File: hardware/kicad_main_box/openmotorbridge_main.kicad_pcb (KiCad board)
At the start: 4 copper layers, 85 x 55 mm, 41 parts, among them J1 DEUTSCH_DTM12_IDC_HEADER, J2 MicroSD_Card, J3 USB2_IDC_HEADER_9PIN, J4 RGB_LED_3PIN, J5 PWR_BAT_NTC_4PIN, SW1 SW_PAIR_RESET, U1 LM5164-Q1, U10 SX1262IMLTRT, U11 TPS7A0533_LDO, U2 ESP32-S3-WROOM-1U-N16R8, U3 ES8388_Codec, U5 BMI270_IMU, U6 TCAN334G, U8 DW3110, U9 QCC3084_BT54_AUDIO, Y1_UWB 38.4MHz

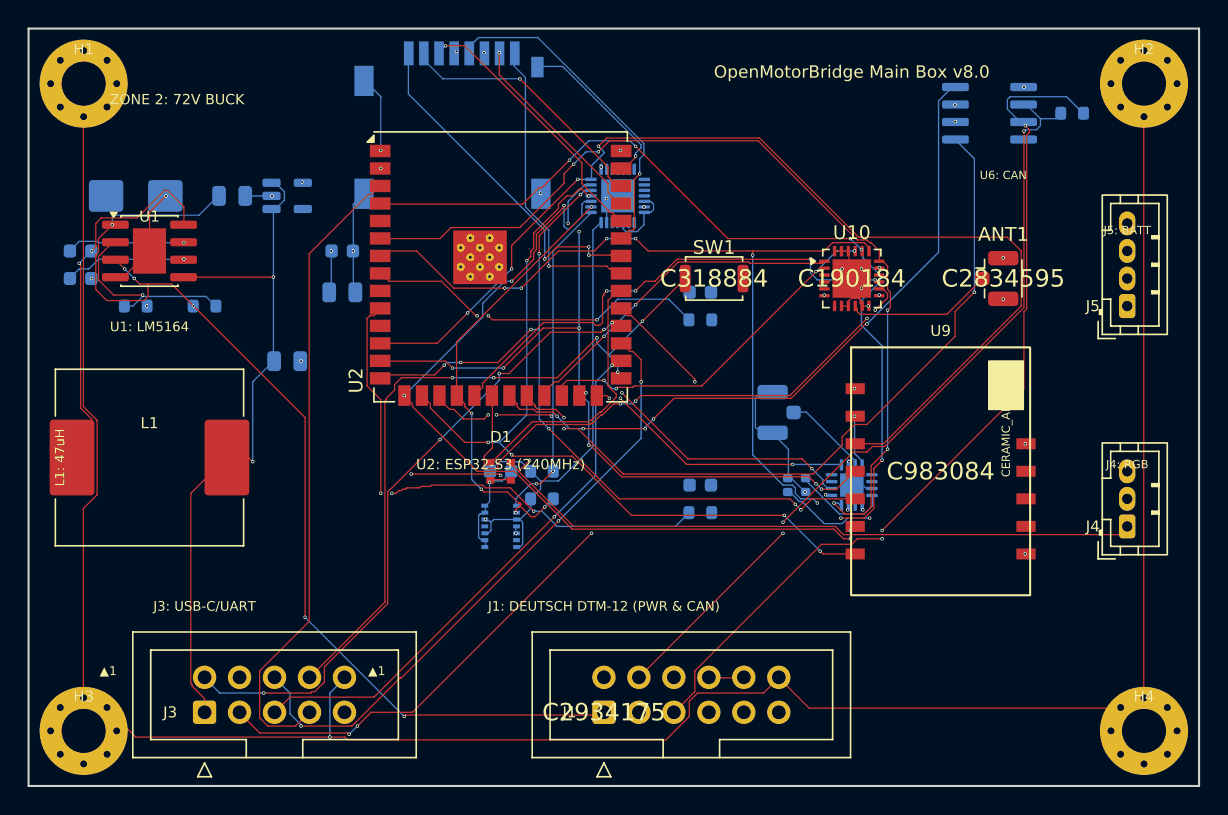
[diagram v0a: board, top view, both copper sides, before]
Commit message: feat: sync re-routed PCBAs (01, 03, 07, 08, 10), manufacturing packages, 3D renders & docs
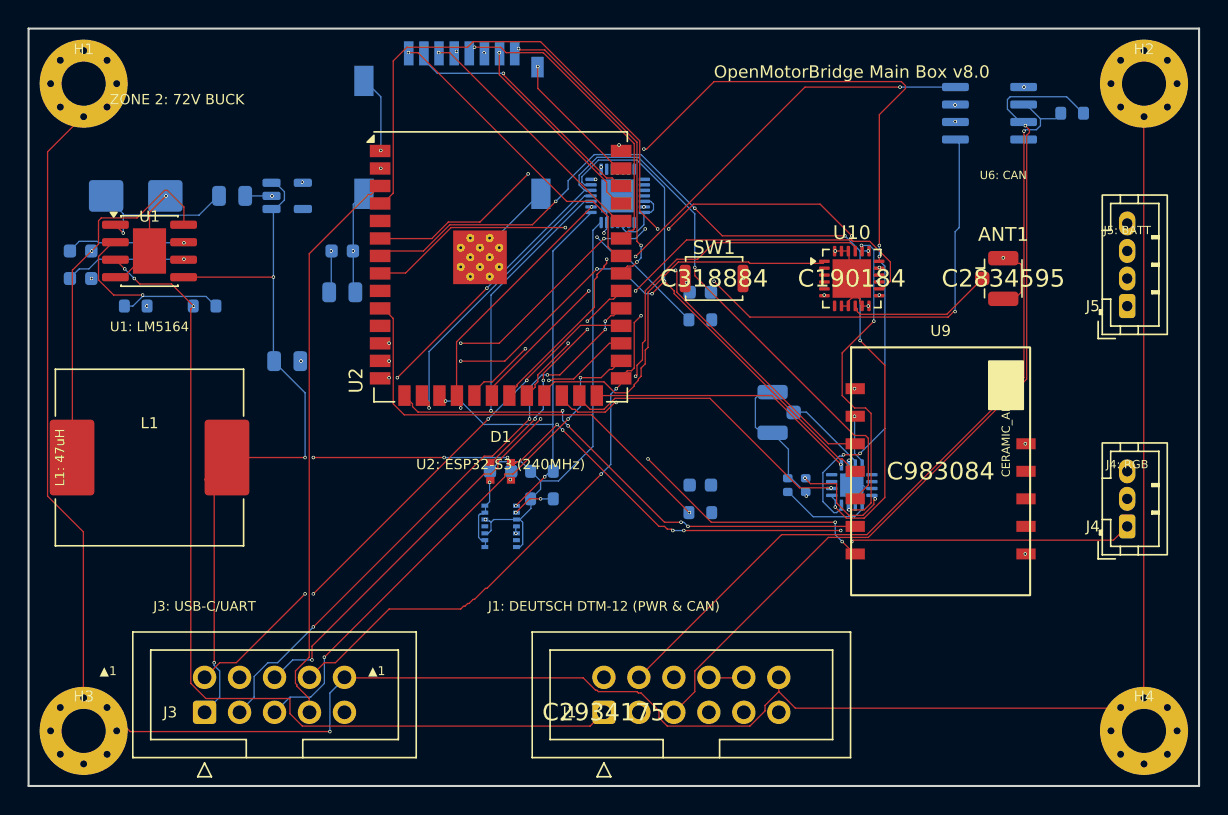
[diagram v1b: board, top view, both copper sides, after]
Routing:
- net I2S_MCLK: track 78.9 -> 50.1 mm, vias 4 -> 6
- net SPI_SCK: track 65.1 -> 79.7 mm, vias 7 -> 6
- net SPI_MISO: track 66.5 -> 78.9 mm, vias 5 -> 6
- net USB_D_P: track 54.2 -> 42.4 mm, vias 4 -> 5
- net GND_PWR: track 88.8 -> 80.3 mm, vias 26 -> 23
- net UART_RXD0: track 45.4 -> 37.3 mm
- net CAN_TX: track 50.3 -> 42.8 mm, vias 5 -> 3
- net ESP_BOOT: track 51.5 -> 44.0 mm, vias 5 -> 4
- net PORT2_KEY_MCU: track 38.8 -> 32.0 mm, vias 3 -> 1
- net USB_D_N: track 47.6 -> 40.9 mm, vias 5 -> 4
- net I2S_DOUT: track 61.8 -> 55.9 mm
- net ESP_EN: track 46.7 -> 40.8 mm
- net LORA_BUSY: track 41.3 -> 36.2 mm, vias 4 -> 2
- net CAN_RX: track 54.0 -> 49.0 mm
- net LORA_NSS: track 25.9 -> 30.4 mm, vias 4 -> 2
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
